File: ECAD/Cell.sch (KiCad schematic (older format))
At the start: 0 parts

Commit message: Cell level and pack level protections, and charge balancing
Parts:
- added BT?: 18650, symbol Device:Battery_Cell
- added C?: 0.1uF, symbol Device:C
- added Q? (x2): Si4186DY, Package_SO:SOIC-8_3.9x4.9mm_P1.27mm, symbol Transistor_FET:Si4162DY
- added R?: 2.7K, symbol Device:R
- added R?: 330R, symbol Device:R
- added U?: AP9101CK, Package_TO_SOT_SMD:SOT-23-5, symbol Battery_Management:AP9101CK
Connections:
- new net: BT?.2 (-), C?.2, Q?.1 (S), Q?.2 (S), Q?.3 (S), U?.3 (VSS)
- new net: R?.1, U?.1 (VM)
- new net: C?.1, R?.2, U?.2 (VDD)
- new net: Q?.4 (G), U?.4 (DO)
- new net: Q?.4 (G), U?.5 (CO)
- new net: Q?.5 (D), Q?.5 (D), Q?.6 (D), Q?.6 (D), Q?.7 (D), Q?.7 (D), Q?.8 (D), Q?.8 (D)
- new net +: BT?.1 (+), R?.1
- new net -: Q?.1 (S), Q?.2 (S), Q?.3 (S), R?.2
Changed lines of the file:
@@
 $Descr A4 11693 8268
 encoding utf-8
-Sheet 3 8
+Sheet 3 10
 Title ""
 Date ""
@@
 Comment4 ""
 $EndDescr
+$Comp
+L Device:Battery_Cell BT?
+U 1 1 61C425E9
+P 4850 3600
+AR Path="/61BD4B7D/61C425E9" Ref="BT?"  Part="1"
+AR Path="/61BD4B7D/61C40A6C/61C425E9" Ref="BT?"  Part="1"
+AR Path="/61BD4B7D/61C444F3/61C425E9" Ref="BT?"  Part="1"
+AR Path="/61BD4B7D/61C44BC0/61C425E9" Ref="BT?"  Part="1"
+AR Path="/61BD4B7D/61C44F8A/61C425E9" Ref="BT?"  Part="1"
+F 0 "BT?" H 4600 3700 50  0000 L CNN
+F 1 "18650" H 4500 3600 50  0000 L CNN
+F 2 "" V 4850 3660 50  0001 C CNN
+F 3 "~" V 4850 3660 50  0001 C CNN
+	1    4850 3600
+	1    0    0    -1
+$EndComp
+$Comp
+L Battery_Management:AP9101CK U?
+U 1 1 61C425EF
+P 5750 3550
+AR Path="/61BD4B7D/61C425EF" Ref="U?"  Part="1"
+AR Path="/61BD4B7D/61C40A6C/61C425EF" Ref="U?"  Part="1"
+AR Path="/61BD4B7D/61C444F3/61C425EF" Ref="U?"  Part="1"
+AR Path="/61BD4B7D/61C44BC0/61C425EF" Ref="U?"  Part="1"
+AR Path="/61BD4B7D/61C44F8A/61C425EF" Ref="U?"  Part="1"
+F 0 "U?" H 5750 4031 50  0000 C CNN
+F 1 "AP9101CK" H 5750 3940 50  0000 C CNN
+F 2 "Package_TO_SOT_SMD:SOT-23-5" H 5700 3550 50  0001 C CNN
+F 3 "https://www.diodes.com/assets/Datasheets/AP9101C.pdf" H 5750 3600 50  0001 C CNN
+	1    5750 3550
+	1    0    0    -1
+$EndComp
+Wire Wire Line
+	4850 3700 4850 3950
+Wire Wire Line
+	4850 3950 5150 3950
+Wire Wire Line
+	5750 3950 5750 3850
+$Comp
+L Transistor_FET:Si4162DY Q?
+U 1 1 61C425F8
+P 6250 3850
+AR Path="/61BD4B7D/61C425F8" Ref="Q?"  Part="1"
+AR Path="/61BD4B7D/61C40A6C/61C425F8" Ref="Q?"  Part="1"
+AR Path="/61BD4B7D/61C444F3/61C425F8" Ref="Q?"  Part="1"
+AR Path="/61BD4B7D/61C44BC0/61C425F8" Ref="Q?"  Part="1"
+AR Path="/61BD4B7D/61C44F8A/61C425F8" Ref="Q?"  Part="1"
+F 0 "Q?" V 6600 3850 50  0000 C CNN
+F 1 "Si4186DY" V 6500 3850 50  0000 C CNN
+F 2 "Package_SO:SOIC-8_3.9x4.9mm_P1.27mm" H 6450 3750 50  0001 L CNN
+F 3 "http://www.vishay.com/docs/68967/si4162dy.pdf" H 6250 3850 50  0001 L CNN
+	1    6250 3850
+	0    1    1    0
+$EndComp
+Wire Wire Line
+	6250 3650 6150 3650
+Wire Wire Line
+	5750 3950 6050 3950
+Connection ~ 5750 3950
+$Comp
+L Transistor_FET:Si4162DY Q?
+U 1 1 61C42601
+P 6650 3850
+AR Path="/61BD4B7D/61C42601" Ref="Q?"  Part="1"
+AR Path="/61BD4B7D/61C40A6C/61C42601" Ref="Q?"  Part="1"
+AR Path="/61BD4B7D/61C444F3/61C42601" Ref="Q?"  Part="1"
+AR Path="/61BD4B7D/61C44BC0/61C42601" Ref="Q?"  Part="1"
+AR Path="/61BD4B7D/61C44F8A/61C42601" Ref="Q?"  Part="1"
+F 0 "Q?" V 7000 3850 50  0000 C CNN
+F 1 "Si4186DY" V 6900 3850 50  0000 C CNN
+F 2 "Package_SO:SOIC-8_3.9x4.9mm_P1.27mm" H 6850 3750 50  0001 L CNN
+F 3 "http://www.vishay.com/docs/68967/si4162dy.pdf" H 6650 3850 50  0001 L CNN
+	1    6650 3850
+	0    -1   1    0
+$EndComp
+Wire Wire Line
+	6650 3650 6650 3450
+Wire Wire Line
+	6650 3450 6150 3450
+Wire Wire Line
+	5350 3550 5350 3200
+Wire Wire Line
+	5350 3200 6900 3200
+$Comp
+L Device:R R?
+U 1 1 61C4260B
+P 6900 3700
+AR Path="/61BD4B7D/61C4260B" Ref="R?"  Part="1"
+AR Path="/61BD4B7D/61C40A6C/61C4260B" Ref="R?"  Part="1"
+AR Path="/61BD4B7D/61C444F3/61C4260B" Ref="R?"  Part="1"
+AR Path="/61BD4B7D/61C44BC0/61C4260B" Ref="R?"  Part="1"
+AR Path="/61BD4B7D/61C44F8A/61C4260B" Ref="R?"  Part="1"
+F 0 "R?" H 6950 3700 50  0000 L CNN
+F 1 "2.7K" V 6900 3700 50  0000 C CNN
+F 2 "" V 6830 3700 50  0001 C CNN
+F 3 "~" H 6900 3700 50  0001 C CNN
+	1    6900 3700
+	1    0    0    -1
+$EndComp
+Wire Wire Line
+	6900 3200 6900 3550
+Wire Wire Line
+	6900 3850 6900 3950
+Wire Wire Line
+	6900 3950 6850 3950
+Connection ~ 6900 3950
+Wire Wire Line
+	4850 3000 7050 3000
+Wire Wire Line
+	6900 3950 7050 3950
+Wire Wire Line
+	4850 3000 4850 3250
+$Comp
+L Device:R R?
+U 1 1 61C42618
+P 5000 3250
+AR Path="/61BD4B7D/61C42618" Ref="R?"  Part="1"
+AR Path="/61BD4B7D/61C40A6C/61C42618" Ref="R?"  Part="1"
+AR Path="/61BD4B7D/61C444F3/61C42618" Ref="R?"  Part="1"
+AR Path="/61BD4B7D/61C44BC0/61C42618" Ref="R?"  Part="1"
+AR Path="/61BD4B7D/61C44F8A/61C42618" Ref="R?"  Part="1"
+F 0 "R?" V 5100 3200 50  0000 L CNN
+F 1 "330R" V 5000 3250 50  0000 C CNN
+F 2 "" V 4930 3250 50  0001 C CNN
+F 3 "~" H 5000 3250 50  0001 C CNN
+	1    5000 3250
+	0    -1   -1   0
+$EndComp
+Connection ~ 4850 3250
+Wire Wire Line
+	4850 3250 4850 3400
+$Comp
+L Device:C C?
+U 1 1 61C42620
+P 5150 3400
+AR Path="/61BD4B7D/61C42620" Ref="C?"  Part="1"
+AR Path="/61BD4B7D/61C40A6C/61C42620" Ref="C?"  Part="1"
+AR Path="/61BD4B7D/61C444F3/61C42620" Ref="C?"  Part="1"
+AR Path="/61BD4B7D/61C44BC0/61C42620" Ref="C?"  Part="1"
+AR Path="/61BD4B7D/61C44F8A/61C42620" Ref="C?"  Part="1"
+F 0 "C?" H 5150 3500 50  0000 L CNN
+F 1 "0.1uF" H 5150 3300 50  0000 L CNN
+F 2 "" H 5188 3250 50  0001 C CNN
+F 3 "~" H 5150 3400 50  0001 C CNN
+	1    5150 3400
+	1    0    0    -1
+$EndComp
+Wire Wire Line
+	5150 3550 5150 3950
+Connection ~ 5150 3950
+Wire Wire Line
+	5150 3950 5750 3950
+Wire Wire Line
+	5150 3250 5750 3250
+Connection ~ 5150 3250
+Text HLabel 7050 3950 2    50   Input ~ 0
+-
+Text HLabel 7050 3000 2    50   Input ~ 0
++
 $EndSCHEMATC

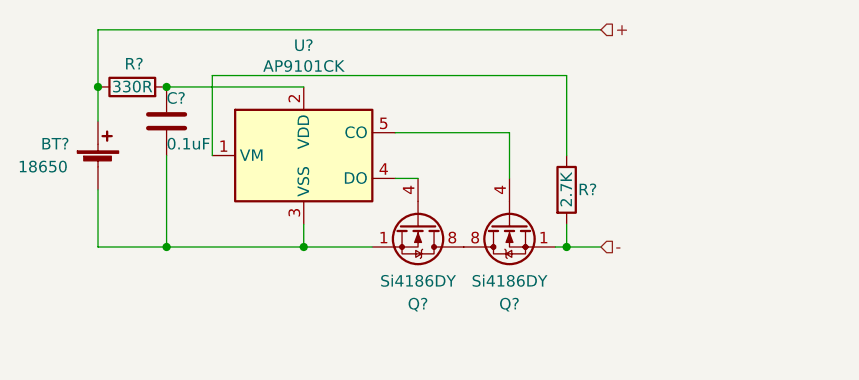
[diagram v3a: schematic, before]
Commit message: revamp solar conditioning, use lt3652 instead of homebrew buck converter
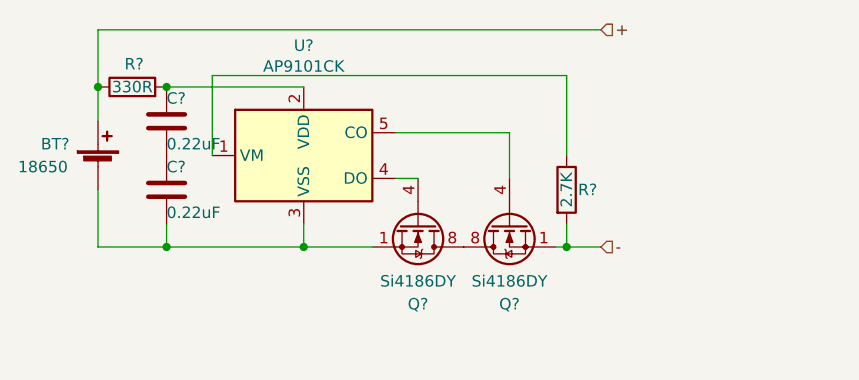
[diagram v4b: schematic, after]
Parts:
- added C?: 0.22uF, symbol Device:C
- C?: value 0.1uF -> 0.22uF
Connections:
- net at BT?.2 (-), Q?.1 (S), Q?.2 (S)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: now also C?.2; no longer C?.2
- new net: C?.1, C?.2
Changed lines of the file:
@@
 	4850 3700 4850 3950
-Wire Wire Line
-	4850 3950 5150 3950
 Wire Wire Line
 	5750 3950 5750 3850
@@
 AR Path="/61BD4B7D/61C44F8A/61C42620" Ref="C?"  Part="1"
 F 0 "C?" H 5150 3500 50  0000 L CNN
-F 1 "0.1uF" H 5150 3300 50  0000 L CNN
+F 1 "0.22uF" H 5150 3300 50  0000 L CNN
 F 2 "" H 5188 3250 50  0001 C CNN
 F 3 "~" H 5150 3400 50  0001 C CNN
@@
 	1    0    0    -1
 $EndComp
-Wire Wire Line
-	5150 3550 5150 3950
-Connection ~ 5150 3950
-Wire Wire Line
-	5150 3950 5750 3950
 Wire Wire Line
 	5150 3250 5750 3250
@@
 Text HLabel 7050 3000 2    50   Input ~ 0
 +
+$Comp
+L Device:C C?
+U 1 1 61CA82AB
+P 5150 3700
+AR Path="/61BD4B7D/61CA82AB" Ref="C?"  Part="1"
+AR Path="/61BD4B7D/61C40A6C/61CA82AB" Ref="C?"  Part="1"
+AR Path="/61BD4B7D/61C444F3/61CA82AB" Ref="C?"  Part="1"
+AR Path="/61BD4B7D/61C44BC0/61CA82AB" Ref="C?"  Part="1"
+AR Path="/61BD4B7D/61C44F8A/61CA82AB" Ref="C?"  Part="1"
+F 0 "C?" H 5150 3800 50  0000 L CNN
+F 1 "0.22uF" H 5150 3600 50  0000 L CNN
+F 2 "" H 5188 3550 50  0001 C CNN
+F 3 "~" H 5150 3700 50  0001 C CNN
+	1    5150 3700
+	1    0    0    -1
+$EndComp
+Wire Wire Line
+	4850 3950 5150 3950
+Wire Wire Line
+	5150 3850 5150 3950
+Connection ~ 5150 3950
+Wire Wire Line
+	5150 3950 5750 3950
 $EndSCHEMATC

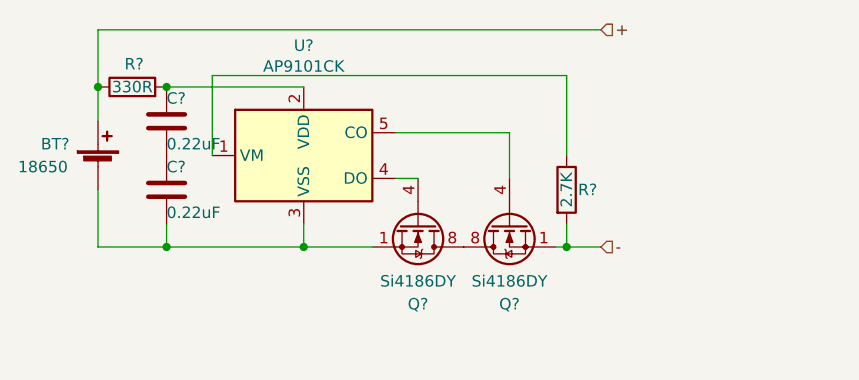
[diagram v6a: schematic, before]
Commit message: spec out new cell protection IC and mosfets, figured out current limit calculation
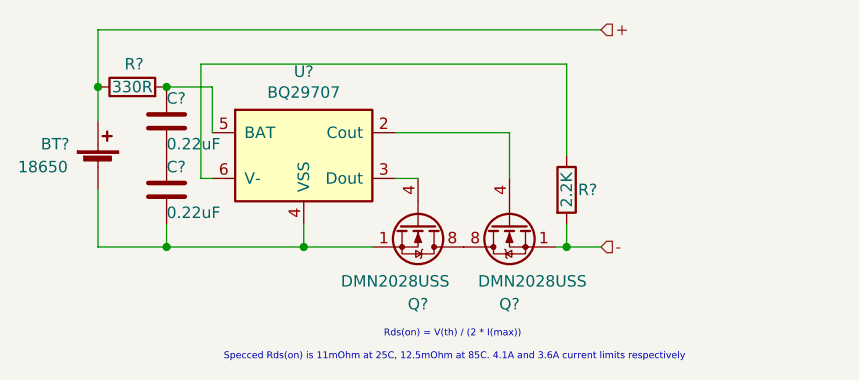
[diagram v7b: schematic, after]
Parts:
- removed U?: AP9101CK, Package_TO_SOT_SMD:SOT-23-5, symbol Battery_Management:AP9101CK
- added U?: BQ29707, Package_SON:WSON-6_1.5x1.5mm_P0.5mm, symbol Battery_Management:BQ297xy
- Q? (x2): value Si4186DY -> DMN2028USS
- R?: value 2.7K -> 2.2K
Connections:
- net at BT?.2 (-), C?.2, Q?.1 (S)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: now also U?.4 (VSS)
- net at R?.1: now also U?.6 (V-)
- net at C?.1, R?.2: now also U?.5 (BAT)
- net at Q?.4 (G): now also U?.3 (Dout)
- net at Q?.4 (G): now also U?.2 (Cout)
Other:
- note added: "Rds(on) = V(th) / (2 * I(max))"
- note added: "Specced Rds(on) is 11mOhm at 25C, 12.5mOhm at 85C. 4.1A and 3.6A current limits respectively"
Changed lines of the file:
@@
-	1    0    0    -1
-$EndComp
-$Comp
-L Battery_Management:AP9101CK U?
-U 1 1 61C425EF
-P 5750 3550
-AR Path="/61BD4B7D/61C425EF" Ref="U?"  Part="1"
-AR Path="/61BD4B7D/61C40A6C/61C425EF" Ref="U?"  Part="1"
-AR Path="/61BD4B7D/61C444F3/61C425EF" Ref="U?"  Part="1"
-AR Path="/61BD4B7D/61C44BC0/61C425EF" Ref="U?"  Part="1"
-AR Path="/61BD4B7D/61C44F8A/61C425EF" Ref="U?"  Part="1"
-F 0 "U?" H 5750 4031 50  0000 C CNN
-F 1 "AP9101CK" H 5750 3940 50  0000 C CNN
-F 2 "Package_TO_SOT_SMD:SOT-23-5" H 5700 3550 50  0001 C CNN
-F 3 "https://www.diodes.com/assets/Datasheets/AP9101C.pdf" H 5750 3600 50  0001 C CNN
-	1    5750 3550
 	1    0    0    -1
 $EndComp
@@
 AR Path="/61BD4B7D/61C44F8A/61C425F8" Ref="Q?"  Part="1"
 F 0 "Q?" V 6600 3850 50  0000 C CNN
-F 1 "Si4186DY" V 6500 3850 50  0000 C CNN
+F 1 "DMN2028USS" V 6500 3750 50  0000 C CNN
 F 2 "Package_SO:SOIC-8_3.9x4.9mm_P1.27mm" H 6450 3750 50  0001 L CNN
 F 3 "http://www.vishay.com/docs/68967/si4162dy.pdf" H 6250 3850 50  0001 L CNN
@@
 AR Path="/61BD4B7D/61C44F8A/61C42601" Ref="Q?"  Part="1"
 F 0 "Q?" V 7000 3850 50  0000 C CNN
-F 1 "Si4186DY" V 6900 3850 50  0000 C CNN
+F 1 "DMN2028USS" V 6900 3750 50  0000 C CNN
 F 2 "Package_SO:SOIC-8_3.9x4.9mm_P1.27mm" H 6850 3750 50  0001 L CNN
 F 3 "http://www.vishay.com/docs/68967/si4162dy.pdf" H 6650 3850 50  0001 L CNN
@@
 Wire Wire Line
 	6650 3450 6150 3450
-Wire Wire Line
-	5350 3550 5350 3200
-Wire Wire Line
-	5350 3200 6900 3200
 $Comp
 L Device:R R?
@@
 AR Path="/61BD4B7D/61C44F8A/61C4260B" Ref="R?"  Part="1"
 F 0 "R?" H 6950 3700 50  0000 L CNN
-F 1 "2.7K" V 6900 3700 50  0000 C CNN
+F 1 "2.2K" V 6900 3700 50  0000 C CNN
 F 2 "" V 6830 3700 50  0001 C CNN
 F 3 "~" H 6900 3700 50  0001 C CNN
@@
 	1    0    0    -1
 $EndComp
-Wire Wire Line
-	6900 3200 6900 3550
 Wire Wire Line
 	6900 3850 6900 3950
@@
 	1    0    0    -1
 $EndComp
-Wire Wire Line
-	5150 3250 5750 3250
-Connection ~ 5150 3250
 Text HLabel 7050 3950 2    50   Input ~ 0
 -
@@
 Wire Wire Line
 	5150 3950 5750 3950
+Text Notes 6100 4350 0    30   ~ 0
+Rds(on) = V(th) / (2 * I(max))
+$Comp
+L Battery_Management:BQ297xy U?
+U 1 1 61D7B95D
+P 5750 3550
+F 0 "U?" H 5750 3917 50  0000 C CNN
+F 1 "BQ29707" H 5750 3826 50  0000 C CNN
+F 2 "Package_SON:WSON-6_1.5x1.5mm_P0.5mm" H 5750 3900 50  0001 C CNN
+F 3 "http://www.ti.com/lit/ds/symlink/bq2970.pdf" H 5500 3750 50  0001 C CNN
+	1    5750 3550
+	1    0    0    -1
+$EndComp
+Wire Wire Line
+	5350 3650 5300 3650
+Wire Wire Line
+	5300 3650 5300 3150
+Wire Wire Line
+	5300 3150 6900 3150
+Wire Wire Line
+	6900 3150 6900 3550
+Wire Wire Line
+	5350 3450 5350 3250
+Wire Wire Line
+	5350 3250 5150 3250
+Connection ~ 5150 3250
+Text Notes 5400 4450 0    30   ~ 0
+Specced Rds(on) is 11mOhm at 25C, 12.5mOhm at 85C. 4.1A and 3.6A current limits respectively
 $EndSCHEMATC
